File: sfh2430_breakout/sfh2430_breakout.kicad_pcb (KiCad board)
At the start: 2 copper layers, 45 x 60.3 mm, 122 parts, among them J1 Landing Pad, J10 Conn_01x01, J11 Conn_01x01, J12 Conn_01x01, J13 Conn_01x01, J2 Landing Pad, J3 Landing Pad, J4 Landing Pad, J5 Conn_01x10, J6 Conn_01x01, J7 Conn_01x01, J8 Conn_01x01, J9 Conn_01x01, U1 LTC2052IS_PBF

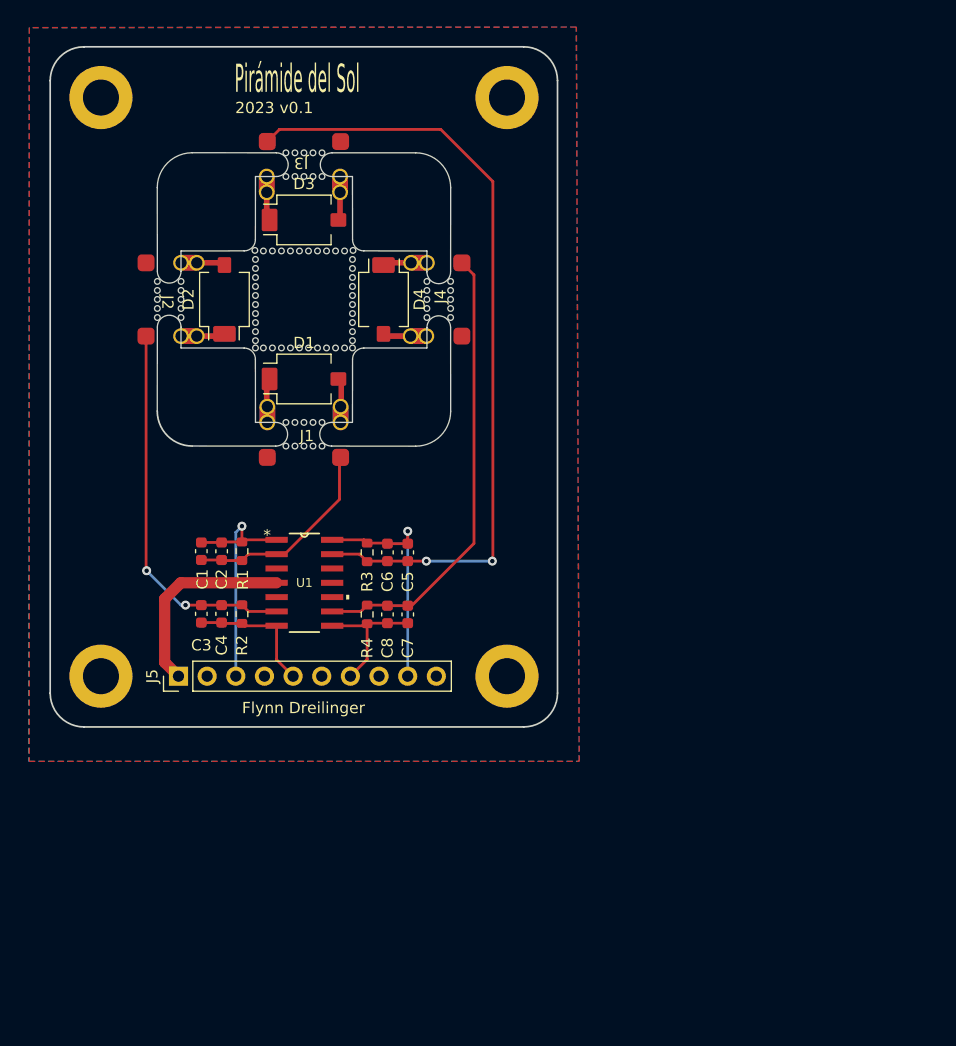
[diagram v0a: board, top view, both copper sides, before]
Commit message: ordered sfh2430 breakout rev 0.1
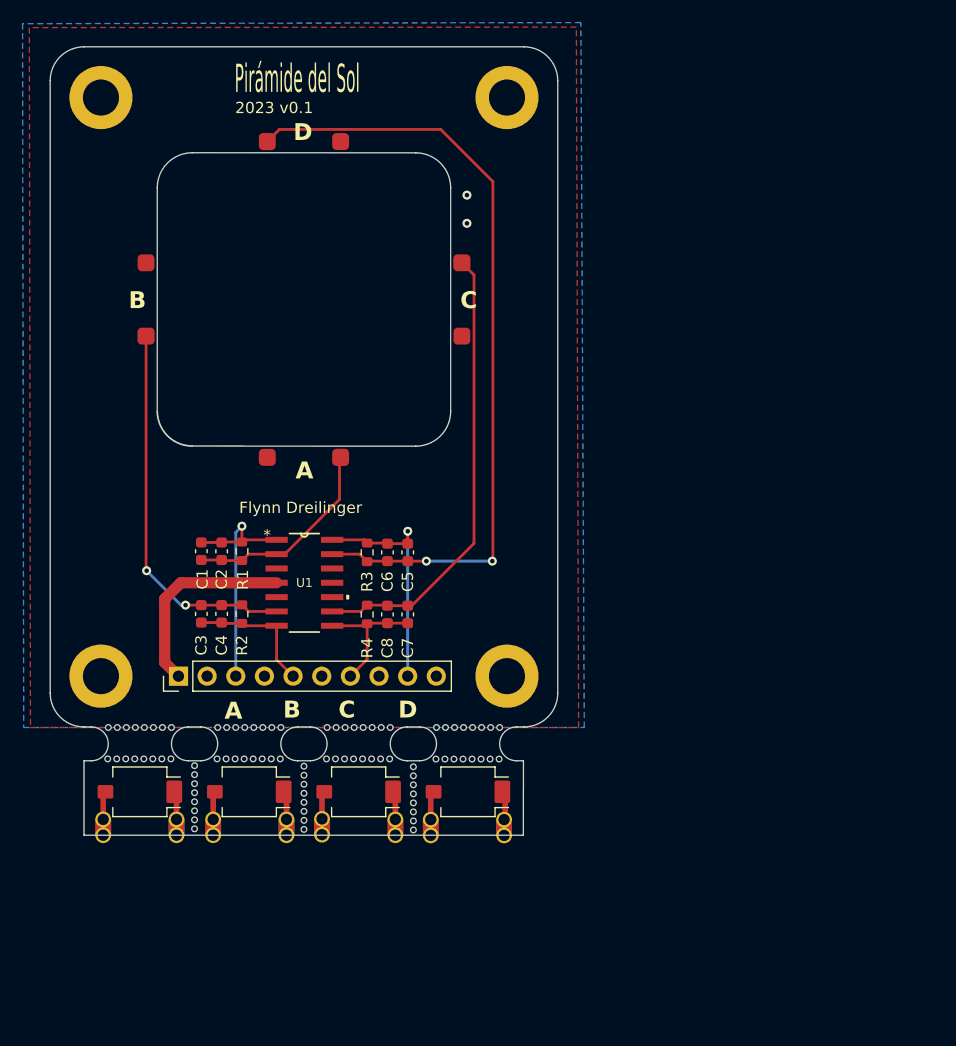
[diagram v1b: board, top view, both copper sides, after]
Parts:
- removed the REF** at (74.4, 79.6)
- removed the REF** at (74.4, 57.8)
- removed the REF** at (77.1, 70.0)
- removed the REF** at (85.8, 67.9)
- removed the REF** at (71.2, 57.8)
- removed the REF** at (74.4, 81.7)
- removed the REF** at (77.1, 73.0)
- removed the REF** at (72.0, 55.7)
- removed the REF** at (76.4, 73.0)
- removed the REF** at (74.0, 64.4)
- removed the REF** at (77.1, 68.3)
- removed the REF** at (73.2, 64.4)
- removed the REF** at (69.2, 64.4)
- removed the REF** at (68.5, 70.8)
- removed the REF** at (68.5, 65.2)
- removed the REF** at (83.7, 67.9)
- removed the REF** at (75.6, 73.0)
- removed the REF** at (61.9, 69.5)
- removed the REF** at (70.0, 73.0)
- removed the REF** at (85.8, 69.5)
- removed the REF** at (73.6, 55.7)
- removed the REF** at (85.8, 67.1)
- removed the REF** at (73.2, 73.0)
- removed the REF** at (72.8, 57.8)
- removed the REF** at (68.5, 71.5)
- removed the REF** at (73.6, 81.7)
- removed the REF** at (68.5, 69.2)
- removed the REF** at (68.5, 66.0)
- removed the REF** at (72.4, 73.0)
- removed the REF** at (77.1, 66.0)
- removed the REF** at (61.9, 67.1)
- removed the REF** at (59.8, 69.5)
- removed the REF** at (70.0, 64.4)
- removed the REF** at (71.2, 79.6)
- removed the REF** at (71.6, 73.0)
- removed the REF** at (72.0, 79.6)
- removed the REF** at (77.2, 64.3)
- removed the REF** at (68.5, 72.3)
- removed the REF** at (71.2, 55.7)
- removed the REF** at (61.9, 70.3)
- removed the REF** at (77.1, 67.5)
- removed the REF** at (68.5, 70.0)
- removed the REF** at (72.0, 81.7)
- removed the REF** at (77.1, 66.8)
- removed the REF** at (77.1, 69.2)
- removed the REF** at (70.8, 64.4)
- removed the REF** at (73.6, 57.8)
- removed the REF** at (59.8, 67.1)
- removed the REF** at (68.5, 68.3)
- removed the REF** at (59.8, 70.3)
- removed the REF** at (74.0, 73.0)
- removed the REF** at (85.8, 70.3)
- removed the REF** at (83.7, 69.5)
- removed the REF** at (72.4, 64.4)
- removed the REF** at (77.1, 70.8)
- removed the REF** at (75.6, 64.4)
- removed the REF** at (70.8, 73.0)
- removed the REF** at (61.9, 68.7)
- removed the REF** at (68.5, 67.5)
- removed the REF** at (74.4, 55.7)
- removed the REF** at (71.6, 64.4)
- removed the REF** at (77.1, 72.3)
- removed the REF** at (59.8, 68.7)
- removed the REF** at (59.8, 67.9)
- removed the REF** at (83.7, 68.7)
- removed the REF** at (72.8, 81.7)
- removed the REF** at (72.8, 55.7)
- removed the REF** at (69.2, 73.0)
- removed the REF** at (73.6, 79.6)
- removed the REF** at (74.8, 73.0)
- removed the REF** at (68.5, 73.0)
- removed the REF** at (68.5, 66.8)
- removed the REF** at (72.0, 57.8)
- removed the REF** at (85.8, 68.7)
- removed the REF** at (61.9, 67.9)
- removed the REF** at (76.4, 64.4)
- removed the REF** at (83.7, 67.1)
- removed the REF** at (74.8, 64.4)
- removed the REF** at (71.2, 81.7)
- removed the REF** at (77.1, 65.2)
- removed the REF** at (83.7, 70.3)
- removed the REF** at (68.5, 64.3)
- removed the REF** at (77.1, 71.5)
- removed the REF** at (72.8, 79.6)
- added REF**: NPTH, NPTH, F.Cu at (87.0, 106.7)
- added REF**: NPTH, NPTH, F.Cu at (72.8, 115.7)
- added REF**: NPTH, NPTH, F.Cu at (66.7, 109.4)
- added REF**: NPTH, NPTH, F.Cu at (82.5, 114.9)
- added REF**: NPTH, NPTH, F.Cu at (75.7, 106.7)
- added REF**: NPTH, NPTH, F.Cu at (60.2, 106.7)
- added REF**: NPTH, NPTH, F.Cu at (58.6, 109.4)
- added REF**: NPTH, NPTH, F.Cu at (77.2, 106.7)
- added REF**: NPTH, NPTH, F.Cu at (63.1, 110.0)
- added REF**: NPTH, NPTH, F.Cu at (61.0, 106.7)
- added REF**: NPTH, NPTH, F.Cu at (77.2, 109.4)
- added REF**: NPTH, NPTH, F.Cu at (68.3, 109.4)
- added REF**: NPTH, NPTH, F.Cu at (79.7, 106.7)
- added REF**: NPTH, NPTH, F.Cu at (57.0, 109.4)
- added REF**: NPTH, NPTH, F.Cu at (84.5, 106.7)
- added REF**: NPTH, NPTH, F.Cu at (63.1, 114.8)
- added REF**: NPTH, NPTH, F.Cu at (87.8, 106.7)
- added REF**: NPTH, NPTH, F.Cu at (89.3, 106.7)
- added REF**: NPTH, NPTH, F.Cu at (78.8, 106.7)
- added REF**: NPTH, NPTH, F.Cu at (67.5, 109.4)
- added REF**: NPTH, NPTH, F.Cu at (72.8, 110.9)
- added REF**: NPTH, NPTH, F.Cu at (58.6, 106.7)
- added REF**: NPTH, NPTH, F.Cu at (82.5, 115.7)
- added REF**: NPTH, NPTH, F.Cu at (82.5, 110.9)
- added REF**: NPTH, NPTH, F.Cu at (76.4, 109.4)
- added REF**: NPTH, NPTH, F.Cu at (79.6, 109.4)
- added REF**: NPTH, NPTH, F.Cu at (90.2, 106.7)
- added REF**: NPTH, NPTH, F.Cu at (66.8, 106.7)
- added REF**: NPTH, NPTH, F.Cu at (84.5, 109.5)
- added REF**: NPTH, NPTH, F.Cu at (86.9, 109.5)
- added REF**: NPTH, NPTH, F.Cu at (82.5, 113.3)
- added REF**: NPTH, NPTH, F.Cu at (60.2, 109.4)
- added REF**: NPTH, NPTH, F.Cu at (63.1, 114.0)
- added REF**: NPTH, NPTH, F.Cu at (63.1, 111.6)
- added REF**: NPTH, NPTH, F.Cu at (57.8, 109.4)
- added REF**: NPTH, NPTH, F.Cu at (82.5, 110.1)
- added REF**: NPTH, NPTH, F.Cu at (85.3, 109.5)
- added REF**: NPTH, NPTH, F.Cu at (72.8, 114.9)
- added REF**: NPTH, NPTH, F.Cu at (69.9, 109.4)
- added REF**: NPTH, NPTH, F.Cu at (74.8, 109.4)
- added REF**: NPTH, NPTH, F.Cu at (69.2, 106.7)
- added REF**: NPTH, NPTH, F.Cu at (57.0, 106.7)
- added REF**: NPTH, NPTH, F.Cu at (63.1, 113.2)
- added REF**: NPTH, NPTH, F.Cu at (57.9, 106.7)
- added REF**: NPTH, NPTH, F.Cu at (66.0, 106.7)
- added REF**: NPTH, NPTH, F.Cu at (72.8, 110.1)
- added REF**: NPTH, NPTH, F.Cu at (56.2, 106.7)
- added REF**: NPTH, NPTH, F.Cu at (55.5, 106.7)
- added REF**: NPTH, NPTH, F.Cu at (74.8, 106.7)
- added REF**: NPTH, NPTH, F.Cu at (65.2, 106.7)
- added REF**: NPTH, NPTH, F.Cu at (69.1, 109.4)
- added REF**: NPTH, NPTH, F.Cu at (68.3, 106.7)
- added REF**: NPTH, NPTH, F.Cu at (88.5, 106.7)
- added REF**: NPTH, NPTH, F.Cu at (86.2, 106.7)
- added REF**: NPTH, NPTH, F.Cu at (87.7, 109.5)
- added REF**: NPTH, NPTH, F.Cu at (72.8, 111.7)
- added REF**: NPTH, NPTH, F.Cu at (55.4, 109.4)
- added REF**: NPTH, NPTH, F.Cu at (72.8, 114.1)
- added REF**: NPTH, NPTH, F.Cu at (82.5, 114.1)
- added REF**: NPTH, NPTH, F.Cu at (78.0, 106.7)
- added REF**: NPTH, NPTH, F.Cu at (63.1, 110.8)
- added REF**: NPTH, NPTH, F.Cu at (59.5, 106.7)
- added REF**: NPTH, NPTH, F.Cu at (65.1, 109.4)
- added REF**: NPTH, NPTH, F.Cu at (59.4, 109.4)
- added REF**: NPTH, NPTH, F.Cu at (88.5, 109.5)
- added REF**: NPTH, NPTH, F.Cu at (70.0, 106.7)
- added REF**: NPTH, NPTH, F.Cu at (82.5, 111.7)
- added REF**: NPTH, NPTH, F.Cu at (61.0, 109.4)
- added REF**: NPTH, NPTH, F.Cu at (80.4, 109.4)
- added REF**: NPTH, NPTH, F.Cu at (63.1, 112.4)
- added REF**: NPTH, NPTH, F.Cu at (76.5, 106.7)
- added REF**: NPTH, NPTH, F.Cu at (63.1, 115.6)
- added REF**: NPTH, NPTH, F.Cu at (80.5, 106.7)
- added REF**: NPTH, NPTH, F.Cu at (56.2, 109.4)
- added REF**: NPTH, NPTH, F.Cu at (70.8, 106.7)
- added REF**: NPTH, NPTH, F.Cu at (70.7, 109.4)
- added REF**: NPTH, NPTH, F.Cu at (78.0, 109.4)
- added REF**: NPTH, NPTH, F.Cu at (90.1, 109.5)
- added REF**: NPTH, NPTH, F.Cu at (65.9, 109.4)
- added REF**: NPTH, NPTH, F.Cu at (86.1, 109.5)
- added REF**: NPTH, NPTH, F.Cu at (72.8, 112.5)
- added REF**: NPTH, NPTH, F.Cu at (89.3, 109.5)
- added REF**: NPTH, NPTH, F.Cu at (67.5, 106.7)
- added REF**: NPTH, NPTH, F.Cu at (78.8, 109.4)
- added REF**: NPTH, NPTH, F.Cu at (85.3, 106.7)
- added REF**: NPTH, NPTH, F.Cu at (75.6, 109.4)
- added REF**: NPTH, NPTH, F.Cu at (82.5, 112.5)
- added REF**: NPTH, NPTH, F.Cu at (72.8, 113.3)
- D1, D2, D3, D4: footprint OptoDevice:Osram_SFH2430 -> adcs:Osram_SFH2430
- moved J11 59.5 mm to (64.8, 116.2), turned to -90 degrees
- moved J10 58.4 mm to (71.2, 116.2), turned to -90 degrees
- moved D3 50.9 mm to (68.0, 112.3), turned to 180 degrees
- moved J12 50.8 mm to (80.9, 116.2), turned to -90 degrees
- moved J9 50.0 mm to (55.0, 114.8), turned to 90 degrees
- moved J13 45.2 mm to (74.4, 116.2), turned to -90 degrees
- moved D2 44.3 mm to (58.2, 112.3), turned to 180 degrees
- moved D4 43.7 mm to (77.7, 112.3), turned to 180 degrees
- moved J8 42.9 mm to (61.5, 114.8), turned to 90 degrees
- moved D1 39.4 mm to (87.3, 112.3), turned to 180 degrees
- moved J6 39.4 mm to (90.5, 114.8)
- moved J7 39.4 mm to (84.0, 114.8)
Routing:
- net GND: vias 0 -> 2
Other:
- board size 45 x 60.3 mm -> 45 x 69.9 mm
- board text added: "A"
- board text added: "B"
- board text added: "C"
- board text added: "D"

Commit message: sfh2400 v2 (flex PCB)
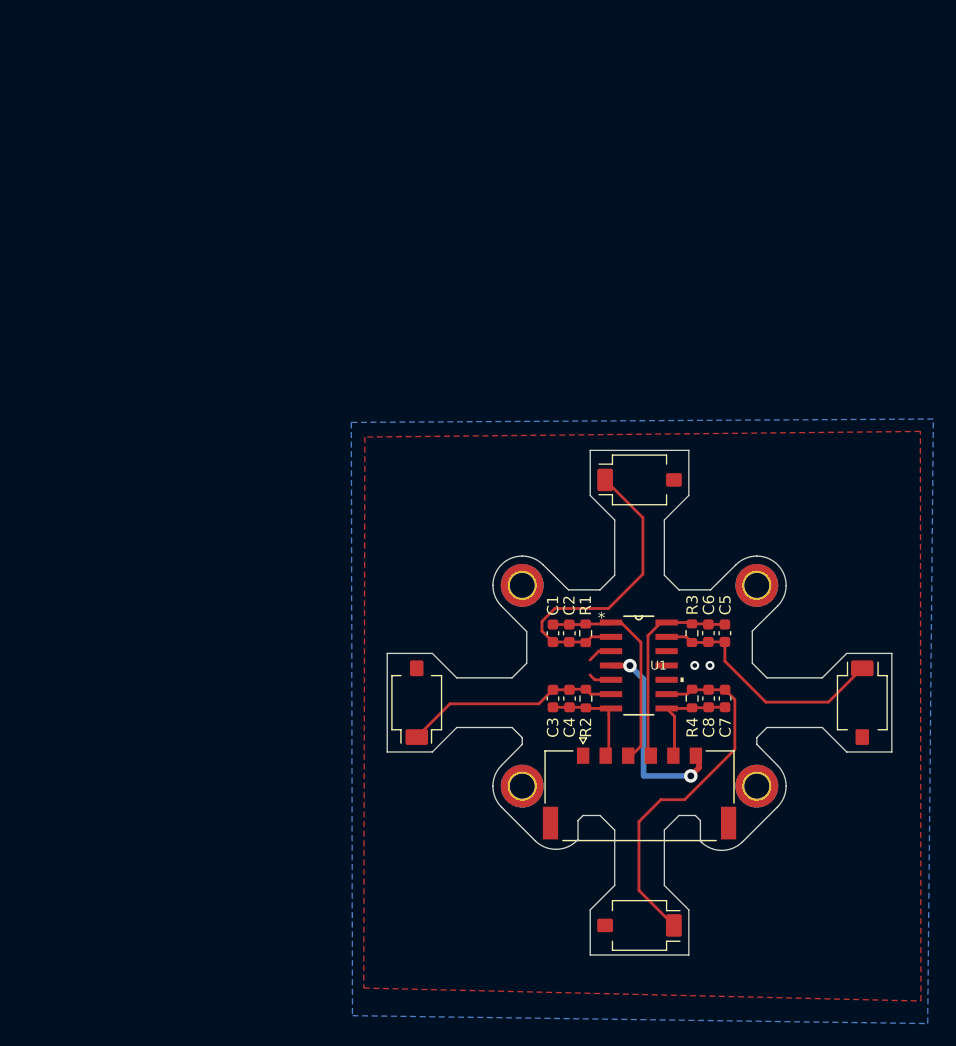
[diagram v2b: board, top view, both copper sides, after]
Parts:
- removed G*** (x2): LOGO, adcs:2ducks
- removed G***: LOGO, adcs:unlimited_ducks_2
- removed G***: LOGO, adcs:sats_pro_shop
- removed H3: MountingHole_Pad, MountingHole:MountingHole_3.2mm_M3_DIN965_Pad
- removed J10, J11, J12, J13, J6, J7, J8, J9: Conn_01x01, adcs:castellated_05mm
- removed J2, J3, J4: Landing Pad, adcs:photodiode_landing_pad
- removed J5: Conn_01x10, Connector_PinHeader_2.54mm:PinHeader_1x10_P2.54mm_Vertical
- removed REF** (x88): NPTH, NPTH
- added locked: MountingHole_Pad, MountingHole:MountingHole_2.2mm_M2_DIN965_Pad_TopBottom, F.Cu at (113.0, 94.0)
- H1, H2, H4: footprint MountingHole:MountingHole_3.2mm_M3_DIN965_Pad -> MountingHole:MountingHole_2.2mm_M2_DIN965_Pad_TopBottom
- J1: value Landing Pad -> Conn_01x06; footprint adcs:photodiode_landing_pad -> sapling:MOLEX_2053380006
- moved H1 57.1 mm to (92.2, 94.0)
- moved D3 54.9 mm to (122.3, 104.5), turned to -90 degrees
- moved J1 42.2 mm to (102.5, 112.7), turned to 180 degrees
- moved H2 38.6 mm to (92.2, 111.8)
- moved C3 32.1 mm to (94.9, 104.1)
- moved C1 32.0 mm to (94.9, 98.3)
- moved C4 31.7 mm to (96.3, 104.1)
- moved C2 31.7 mm to (96.3, 98.3)
- moved D1 31.6 mm to (102.5, 84.7), turned to 0 degrees
- moved R2 31.4 mm to (97.8, 104.1)
- moved R1 31.3 mm to (97.8, 98.3)
- moved U1 30.5 mm to (102.5, 101.2)
- moved R4 29.8 mm to (107.2, 104.1)
- moved R3 29.7 mm to (107.2, 98.3)
- moved C8 29.4 mm to (108.7, 104.1)
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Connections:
- C1 pad 1: Net-(J1-Pin_2) -> /Photodiode 1/IN-
- C1 pad 2: /OUTA -> /OUT1
- C2 pad 1: Net-(J1-Pin_2) -> /Photodiode 1/IN-
- C2 pad 2: /OUTA -> /OUT1
- C3 pad 1: Net-(J2-Pin_2) -> /Photodiode 2/IN-
- C3 pad 2: /OUTB -> /OUT2
- C4 pad 1: Net-(J2-Pin_2) -> /Photodiode 2/IN-
- C4 pad 2: /OUTB -> /OUT2
- C5 pad 1: Net-(J3-Pin_2) -> /Photodiode 4/IN-
- C5 pad 2: /OUTD -> /OUT4
- C6 pad 1: Net-(J3-Pin_2) -> /Photodiode 4/IN-
- C6 pad 2: /OUTD -> /OUT4
- C7 pad 1: Net-(J4-Pin_2) -> /Photodiode 3/IN-
- C7 pad 2: /OUTC -> /OUT3
- C8 pad 1: Net-(J4-Pin_2) -> /Photodiode 3/IN-
- C8 pad 2: /OUTC -> /OUT3
- D1 pad 1: Net-(D1-K) -> /Photodiode 1/IN-
- D1 pad 2: Net-(D1-A) -> GND
- D2 pad 1: Net-(D2-K) -> /Photodiode 2/IN-
- D2 pad 2: Net-(D2-A) -> GND
- D3 pad 1: Net-(D3-K) -> /Photodiode 4/IN-
- D3 pad 2: Net-(D3-A) -> GND
- D4 pad 1: Net-(D4-K) -> /Photodiode 3/IN-
- D4 pad 2: Net-(D4-A) -> GND
- J1 pad 2: Net-(J1-Pin_2) -> /OUT2
- R1 pad 1: Net-(J1-Pin_2) -> /Photodiode 1/IN-
- R1 pad 2: /OUTA -> /OUT1
- R2 pad 1: Net-(J2-Pin_2) -> /Photodiode 2/IN-
- R2 pad 2: /OUTB -> /OUT2
- R3 pad 1: Net-(J3-Pin_2) -> /Photodiode 4/IN-
- R3 pad 2: /OUTD -> /OUT4
- R4 pad 1: Net-(J4-Pin_2) -> /Photodiode 3/IN-
- R4 pad 2: /OUTC -> /OUT3
- U1 pad 1: /OUTA -> /OUT1
- U1 pad 13: Net-(J3-Pin_2) -> /Photodiode 4/IN-
- U1 pad 14: /OUTD -> /OUT4
- U1 pad 2: Net-(J1-Pin_2) -> /Photodiode 1/IN-
- U1 pad 6: Net-(J2-Pin_2) -> /Photodiode 2/IN-
- U1 pad 7: /OUTB -> /OUT2
- U1 pad 8: /OUTC -> /OUT3
- U1 pad 9: Net-(J4-Pin_2) -> /Photodiode 3/IN-
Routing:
- net Net-(J3-Pin_2): track 70.5 -> 0.00 mm, vias 2 -> 0
- net Net-(J4-Pin_2): track 40.4 -> 0.00 mm
- net Net-(J2-Pin_2): track 33.9 -> 0.00 mm, vias 2 -> 0
- net /Photodiode 3/IN-: track 0.00 -> 32.7 mm
- net /Photodiode 1/IN-: track 0.00 -> 28.0 mm
- net /Photodiode 4/IN-: track 0.00 -> 22.0 mm
- net /OUTA: track 21.7 -> 0.00 mm, vias 1 -> 0
- net /OUTD: track 20.8 -> 0.00 mm, vias 1 -> 0
- net /Photodiode 2/IN-: track 0.00 -> 19.2 mm
- net /OUT1: track 0.00 -> 19.0 mm
- net Net-(J1-Pin_2): track 18.3 -> 0.00 mm
- net /OUT4: track 0.00 -> 18.2 mm
- net /OUTC: track 12.1 -> 0.00 mm
- net /OUTB: track 11.9 -> 0.00 mm
- net /OUT3: track 0.00 -> 9.79 mm
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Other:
- board size 45 x 69.9 mm -> 44.7 x 44.7 mm
- board text removed: "2023 v0.1"
- board text removed: "A"
- board text removed: "B"
- board text removed: "C"
- board text removed: "D"
- board text removed: "Flynn Dreilinger"
- board text removed: "Pirámide del Sol"
